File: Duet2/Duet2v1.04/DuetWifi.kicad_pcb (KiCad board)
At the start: 4 copper layers, 100 x 123 mm, 430 parts, among them J1 EXPANSION, J10 E0 MOT, J11 E0 HEAT, J12 E0 TEMP, J13 E1 HEAT, J14 E1 TEMP, J15 uSDHC, J16 CONN_ALT_HEADER, J17 + + - -, J18 + + - -, J19 Z_STOP, J2 FAN2, J20 5V_PS, J21 JTAG, J22 USB, J23 VIN, J24 GND V_IN, J25 FAN0, J26 E2/E3_UART, J27 UART, J28 Probe, J29 FAN1, J3 5V V_FAN VIN, J30 PanelDUE, J31 GND V_IN, J32 Y_STOP, J33 X_STOP, J34 E0_STOP, J35 E1_STOP, J36 Z A, J37 SPI0, J38 ENN, J39 ESP_COMMS, J4 BED HEAT, J40 DIR, J41 STEP, J42 UART, J43 ENN, J44 DIR, J45 STEP, J46 UART, J47 ENN, J48 DIR, J49 STEP, J5 BED TEMP, J50 UART, J51 ENN, J52 DIR, J53 STEP, J54 UART, J55 ENN, J56 DIR, J57 STEP, J6 E1 MOT, J7 Z B, J8 Y MOT, J9 X MOT, M1 FID, M11 LOGO, M2 FID, M3 FID, M4 MOUNTING, M5 MOUNTING, M6 MOUNTING, M7 MOUNTING, M8 LOGO, P1 CONN_SD, P2 CONN_LCD, U1 ATSAM4E8E, U10 MAX31865AAP(SSOP20), U11 74HCT02, U12 74HC74, U13 MAX31865AAP(SSOP20), U16 SN74CB3Q3251, U2 AP7361C-33E-13, U3 A4403, U4 ESP-07/12, U5 TMC2224, U6 TMC2224, U7 TMC2224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

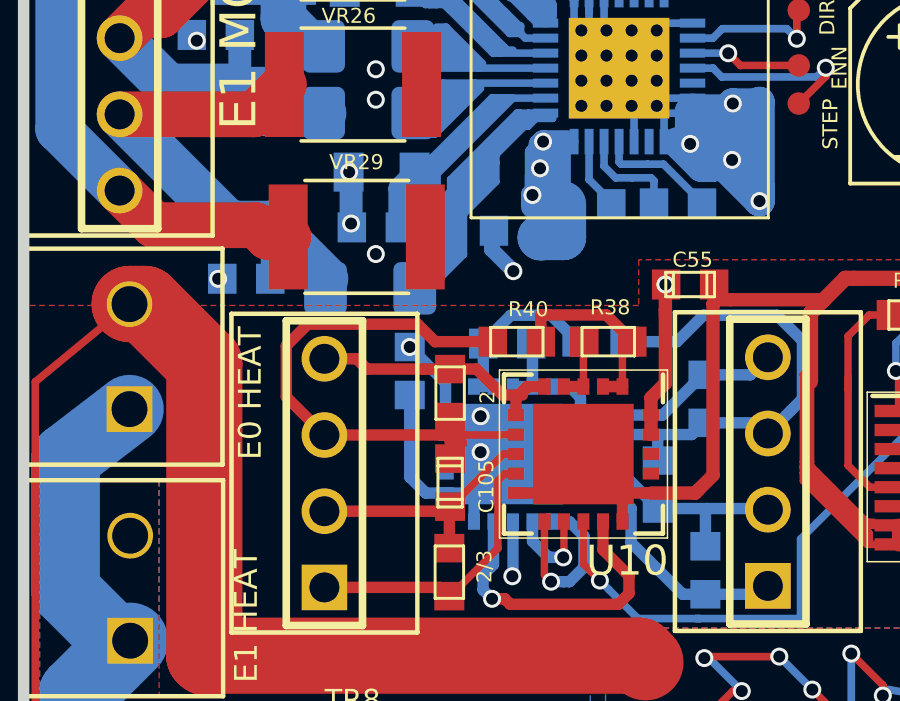
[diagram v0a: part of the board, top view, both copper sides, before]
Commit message: fixed DRC
FIxed DRC errors.
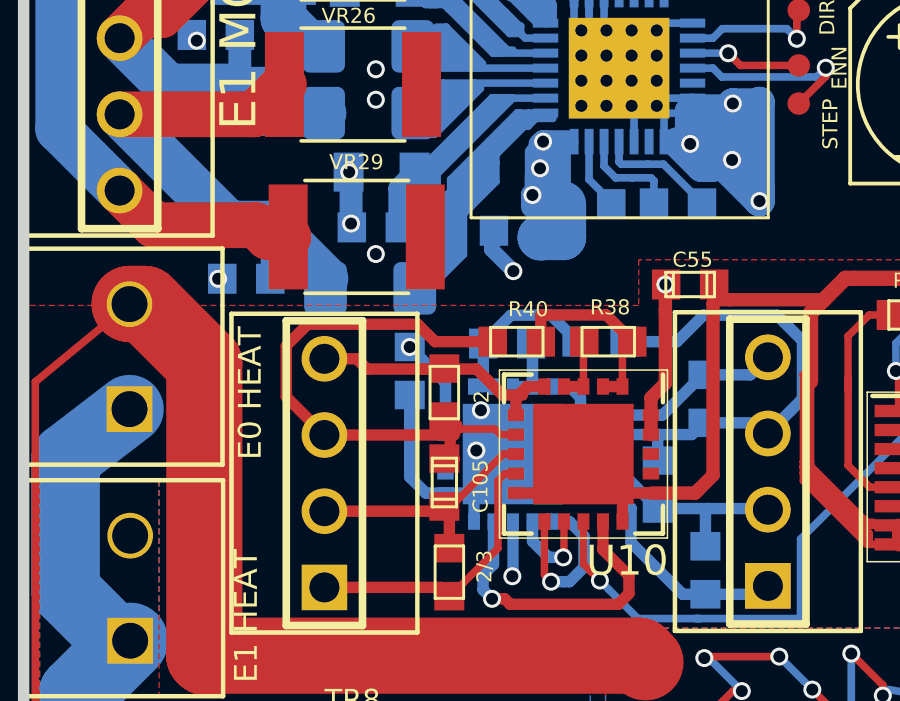
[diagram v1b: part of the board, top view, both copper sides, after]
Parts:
- moved Ju1 0.19 mm to (94.2, 127.6)
- moved C105 0.19 mm to (94.2, 130.6)
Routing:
- net Net-(L25-Pad2): track 46.2 -> 49.4 mm
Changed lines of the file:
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@@
     (thickness 1.6002)
     (drawings 374)
-    (tracks 10011)
+    (tracks 10021)
     (zones 0)
     (modules 430)
@@
   (layers
     (0 Front mixed)
-    (1 Inner3 signal)
+    (1 Inner3 signal hide)
     (2 Inner2 power hide)
-    (31 Back power)
+    (31 Back power hide)
     (35 F.Paste user hide)
-    (36 B.SilkS user)
+    (36 B.SilkS user hide)
     (37 F.SilkS user)
     (38 B.Mask user hide)
@@
   )
   (module complib:C_0603 (layer Front)
-    (at 94.427 130.55998 270)
+    (at 94.234 130.556 270)
     (descr "SMT capacitor, 0603")
     (fp_text reference C105 (at 0.127 -1.2065 270) (layer F.SilkS)
@@
   )
   (module complib:R_0603 (layer Front)
-    (at 94.427 127.57548 90)
+    (at 94.234 127.5588 90)
     (attr smd)
     (fp_text reference Ju1 (at 0.0508 1.0922 90) (layer F.SilkS) hide
@@
   (segment (start 98.7725 130.90748) (end 96.7765 130.87748) (width 0.381) (layer Back) (net 67))
   (segment (start 103.317 124.08298) (end 103.317 124.46398) (width 0.4455) (layer Front) (net 67))
-  (via (at 95.443 128.34747) (size 0.6) (drill 0.4) (layers Front Back) (net 67))
-  (via (at 95.443 129.54398) (size 0.6) (drill 0.4) (layers Front Back) (net 67))
+  (via (at 95.3008 129.4892) (size 0.6) (drill 0.4) (layers Front Back) (net 67))
   (segment (start 101.122 130.90748) (end 102.596952 130.90748) (width 0.4455) (layer Front) (net 67))
   (segment (start 101.122 130.90748) (end 100.172 130.90748) (width 0.381) (layer Front) (net 67))
@@
   (segment (start 97.572 130.90748) (end 98.872 129.60748) (width 0.381) (layer Front) (net 67))
   (segment (start 96.622 130.90748) (end 97.572 130.90748) (width 0.381) (layer Front) (net 67))
+  (via (at 95.4532 128.14587) (size 0.6) (drill 0.4) (layers Front Back) (net 67))
   (segment (start 144.566639 117.078761) (end 144.26692 117.37848) (width 0.254) (layer Front) (net 68))
   (segment (start 145.553855 117.078761) (end 144.566639 117.078761) (width 0.254) (layer Front) (net 68))
@@
   (segment (start 89.474001 128.210481) (end 90.236 128.97248) (width 0.254) (layer Front) (net 284))
   (segment (start 95.8494 125.86098) (end 95.12042 125.86098) (width 0.254) (layer Front) (net 284))
-  (segment (start 94.81308 129.23156) (end 94.554 128.97248) (width 0.381) (layer Front) (net 284))
-  (segment (start 94.554 128.97248) (end 94.808 128.97248) (width 0.381) (layer Front) (net 284))
+  (segment (start 94.6404 128.6256) (end 94.38132 128.36652) (width 0.381) (layer Front) (net 284))
+  (segment (start 94.3356 128.6764) (end 94.5896 128.6764) (width 0.381) (layer Front) (net 284))
   (segment (start 94.554 128.50258) (end 94.427 128.37558) (width 0.381) (layer Front) (net 284))
   (segment (start 94.554 128.97248) (end 94.554 128.50258) (width 0.381) (layer Front) (net 284))
@@
   (segment (start 88.966 127.70248) (end 90.236 128.97248) (width 0.381) (layer Front) (net 284))
   (segment (start 88.966 125.996778) (end 88.966 127.70248) (width 0.381) (layer Front) (net 284))
-  (segment (start 96.082 128.97248) (end 94.554 128.97248) (width 0.25) (layer Front) (net 284))
-  (segment (start 96.097 128.95748) (end 96.082 128.97248) (width 0.25) (layer Front) (net 284))
   (segment (start 96.622 128.95748) (end 96.097 128.95748) (width 0.25) (layer Front) (net 284))
+  (segment (start 96.097 128.95748) (end 95.9104 128.77088) (width 0.25) (layer Front) (net 284))
+  (segment (start 95.9104 128.77088) (end 94.7556 128.77088) (width 0.25) (layer Front) (net 284))
+  (segment (start 94.7556 128.77088) (end 94.554 128.97248) (width 0.25) (layer Front) (net 284))
   (segment (start 94.1095 134.05248) (end 94.4016 134.34458) (width 0.381) (layer Front) (net 285))
   (segment (start 90.236 134.05248) (end 94.1095 134.05248) (width 0.381) (layer Front) (net 285))
@@
   (segment (start 93.792 120.46348) (end 93.792 120.20948) (width 0.254) (layer Back) (net 287))
   (segment (start 93.991 120.65818) (end 93.991 120.64548) (width 0.254) (layer Back) (net 287))
-  (segment (start 92.7506 121.89858) (end 93.991 120.65818) (width 0.254) (layer Back) (net 287))
+  (segment (start 92.7506 121.8396) (end 93.991 120.5992) (width 0.254) (layer Back) (net 287))
   (segment (start 92.7506 121.92398) (end 92.7506 121.89858) (width 0.254) (layer Back) (net 287))
   (segment (start 92.7506 121.92398) (end 92.7506 121.63188) (width 0.254) (layer Back) (net 287))
@@
   (segment (start 93.2475 123.76548) (end 93.2475 122.91298) (width 0.254) (layer Back) (net 321))
   (segment (start 93.552581 122.607899) (end 93.552581 122.49548) (width 0.254) (layer Back) (net 321))
-  (segment (start 93.2475 122.91298) (end 93.552581 122.607899) (width 0.254) (layer Back) (net 321))
+  (segment (start 93.319319 122.936281) (end 93.6244 122.6312) (width 0.254) (layer Back) (net 321))
   (segment (start 93.552581 122.49548) (end 93.552581 122.861899) (width 0.254) (layer Back) (net 321))
   (segment (start 93.552581 121.738665) (end 93.552581 122.49548) (width 0.254) (layer Back) (net 321))
@@
   (segment (start 93.665 121.86048) (end 93.665 122.36848) (width 0.254) (layer Back) (net 321))
   (segment (start 93.665 122.36848) (end 93.665 122.58598) (width 0.254) (layer Back) (net 321))
-  (segment (start 93.2475 123.76548) (end 94.046 122.96698) (width 0.254) (layer Back) (net 321))
   (segment (start 93.9825 121.66998) (end 93.919 121.60648) (width 0.254) (layer Back) (net 321))
   (segment (start 93.9825 123.06698) (end 93.9825 121.66998) (width 0.254) (layer Back) (net 321))
@@
   (segment (start 96.9035 118.67268) (end 96.9035 118.62198) (width 0.254) (layer Back) (net 321))
   (segment (start 96.9035 118.62198) (end 97.1575 118.36798) (width 0.254) (layer Back) (net 321))
+  (segment (start 93.2475 123.10798) (end 93.36868 122.9868) (width 0.25) (layer Back) (net 321))
+  (segment (start 93.2475 124.08298) (end 93.2475 123.10798) (width 0.25) (layer Back) (net 321))
+  (segment (start 93.82298 122.9868) (end 93.92458 123.0884) (width 0.25) (layer Back) (net 321))
+  (segment (start 93.36868 122.9868) (end 93.82298 122.9868) (width 0.25) (layer Back) (net 321))
+  (segment (start 93.92458 123.0884) (end 94.046 122.96698) (width 0.254) (layer Back) (net 321))
+  (segment (start 93.2475 124.08298) (end 93.2475 123.3129) (width 0.25) (layer Back) (net 321))
+  (segment (start 93.4212 123.1392) (end 93.87378 123.1392) (width 0.25) (layer Back) (net 321))
+  (segment (start 93.2475 123.3129) (end 93.4212 123.1392) (width 0.25) (layer Back) (net 321))
+  (segment (start 93.87378 123.1392) (end 93.92458 123.0884) (width 0.254) (layer Back) (net 321))
+  (segment (start 93.2475 123.76548) (end 93.87378 123.1392) (width 0.254) (layer Back) (net 321))
   (segment (start 94.1815 117.24348) (end 93.184 118.24098) (width 0.25) (layer Back) (net 322))
   (segment (start 93.184 118.24098) (end 93.2205 118.24098) (width 0.254) (layer Back) (net 322))
